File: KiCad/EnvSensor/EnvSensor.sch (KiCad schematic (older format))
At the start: 90 parts, among them J1 SWD, J2 I2C, J3 USB_B_Micro, J4 Barrel_Jack, J5 Micro_SD_Card, P1 USB_C_Plug_USB2.0, Q1 IRLML2502, Q2 IRF7404, Q3 SQJB80EP, SW1 SW_Push, SW2 SW_Push, SW3 SW_Push, SW4 SW_Push, U1 STM32L431CCT6, U10 BME280-Module, U11 E-Ink_Waveshare_4.2, U2 MCP73843-4.2, U3 AP9101CK, U4 BME280, U5 SCD30, U6 TPS782-DDC, U7 TPS782-DDC, U8 HIH8121, U9 ESP-12S, Y1 16MHz, Y2 32768/12.5pF

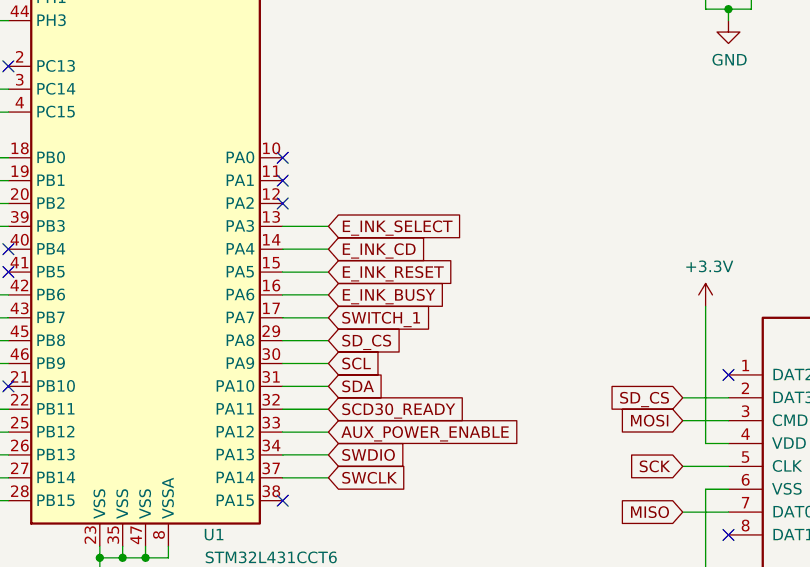
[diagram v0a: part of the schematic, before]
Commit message: Work on pcb v2
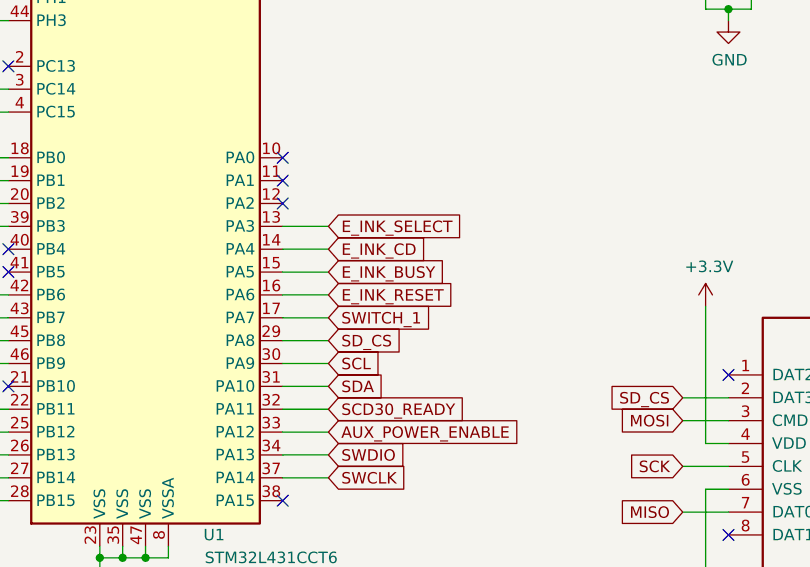
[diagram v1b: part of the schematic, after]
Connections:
- net E_INK_BUSY: now also U1.15 (PA5); no longer U1.16 (PA6)
- net E_INK_RESET: now also U1.16 (PA6); no longer U1.15 (PA5)
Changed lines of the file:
@@
 Text GLabel 5600 10150 2    50   Input ~ 0
 E_INK_CD
+Text GLabel 5600 10350 2    50   Input ~ 0
+E_INK_RESET
 Text GLabel 5600 10250 2    50   Input ~ 0
-E_INK_RESET
-Text GLabel 5600 10350 2    50   Input ~ 0
 E_INK_BUSY
 Wire Wire Line

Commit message: Finishing touches
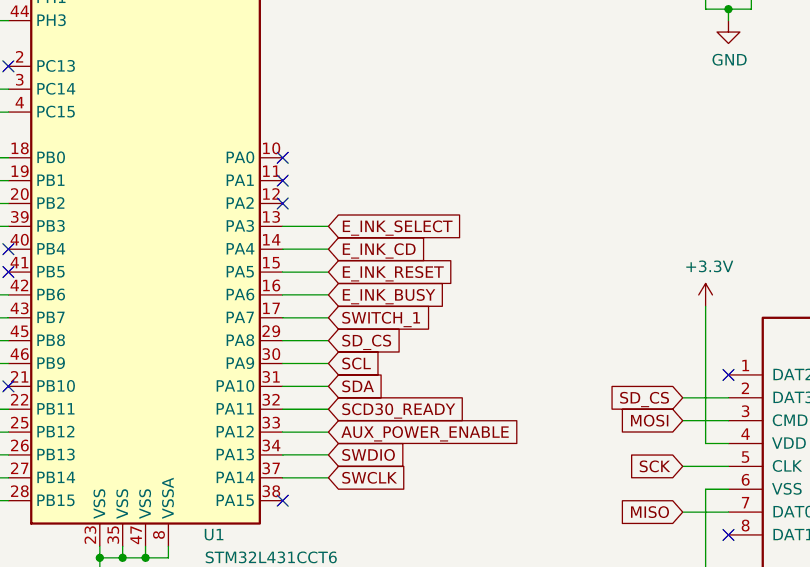
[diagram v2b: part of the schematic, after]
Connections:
- net E_INK_BUSY: now also U1.16 (PA6); no longer U1.15 (PA5)
- net E_INK_RESET: now also U1.15 (PA5); no longer U1.16 (PA6)
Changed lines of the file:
@@
 Text GLabel 5600 10150 2    50   Input ~ 0
 E_INK_CD
-Text GLabel 5600 10350 2    50   Input ~ 0
-E_INK_RESET
-Text GLabel 5600 10250 2    50   Input ~ 0
-E_INK_BUSY
 Wire Wire Line
 	9950 10850 10150 10850
@@
 Wire Wire Line
 	4900 4150 4900 4700
+Text GLabel 5600 10350 2    50   Input ~ 0
+E_INK_BUSY
+Text GLabel 5600 10250 2    50   Input ~ 0
+E_INK_RESET
 $EndSCHEMATC
